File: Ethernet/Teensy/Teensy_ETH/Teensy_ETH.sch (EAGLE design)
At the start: 3 parts, among them M1 TEENSY4.1

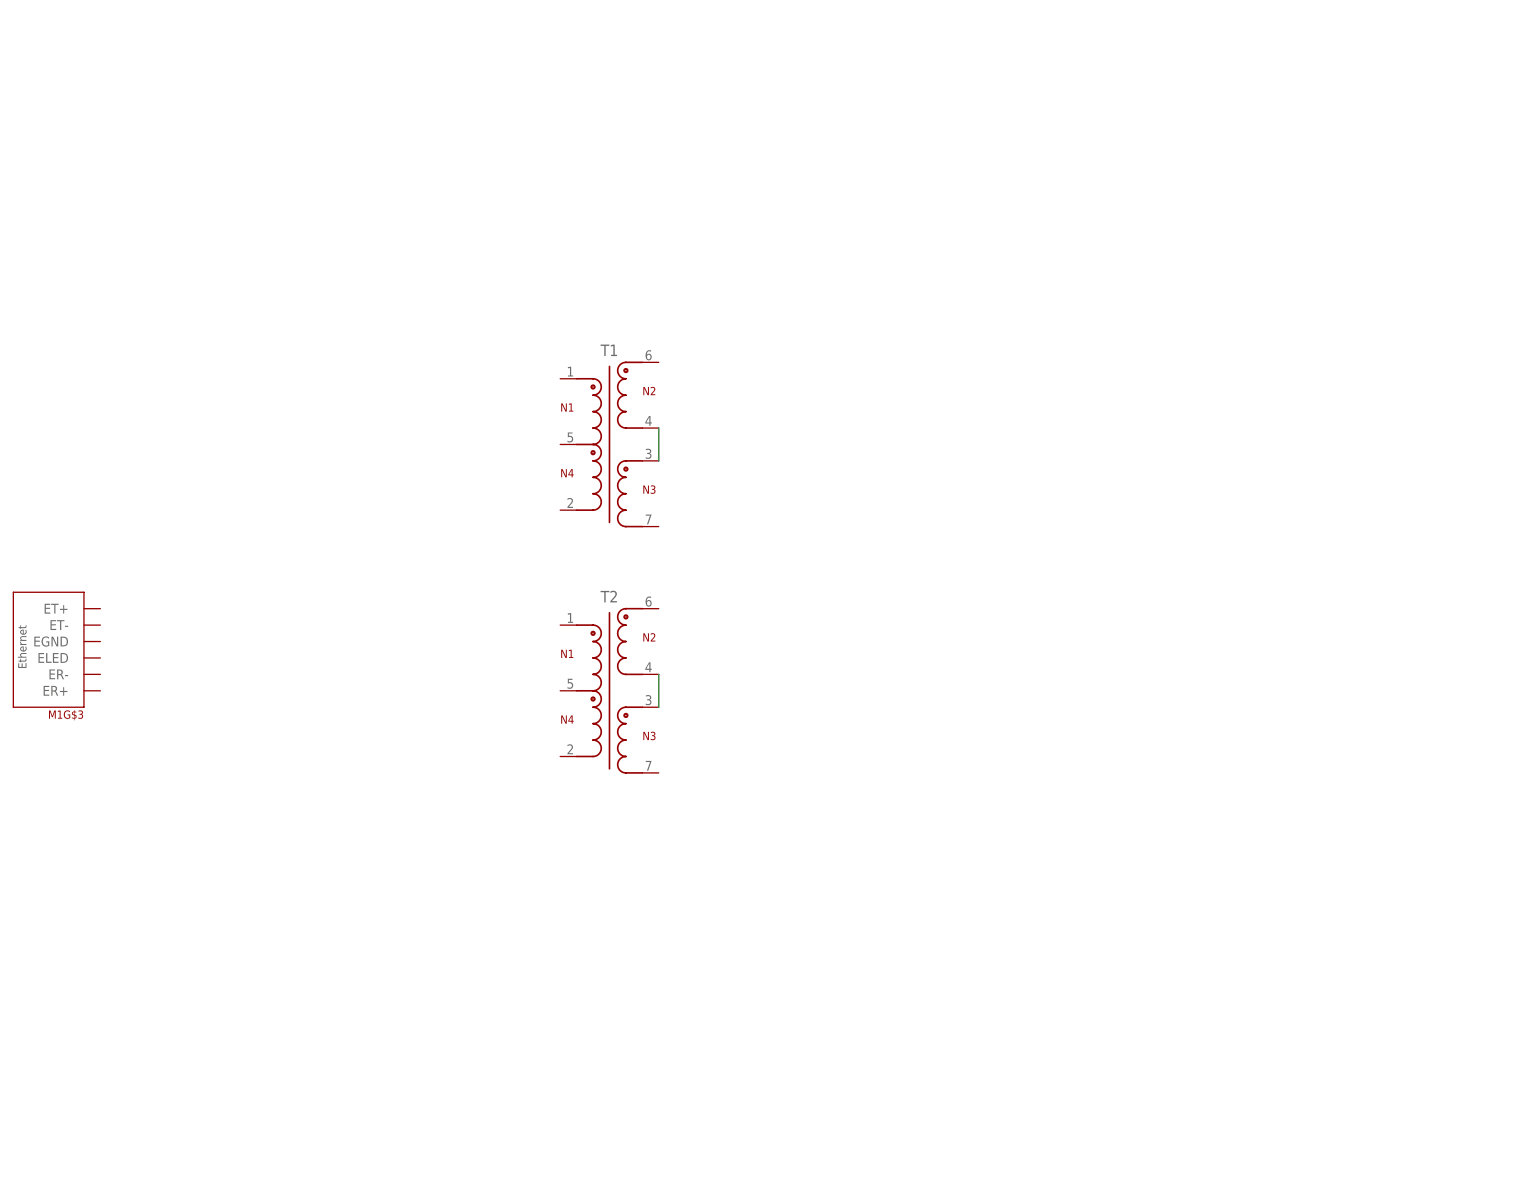
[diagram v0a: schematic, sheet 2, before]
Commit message: sicherung
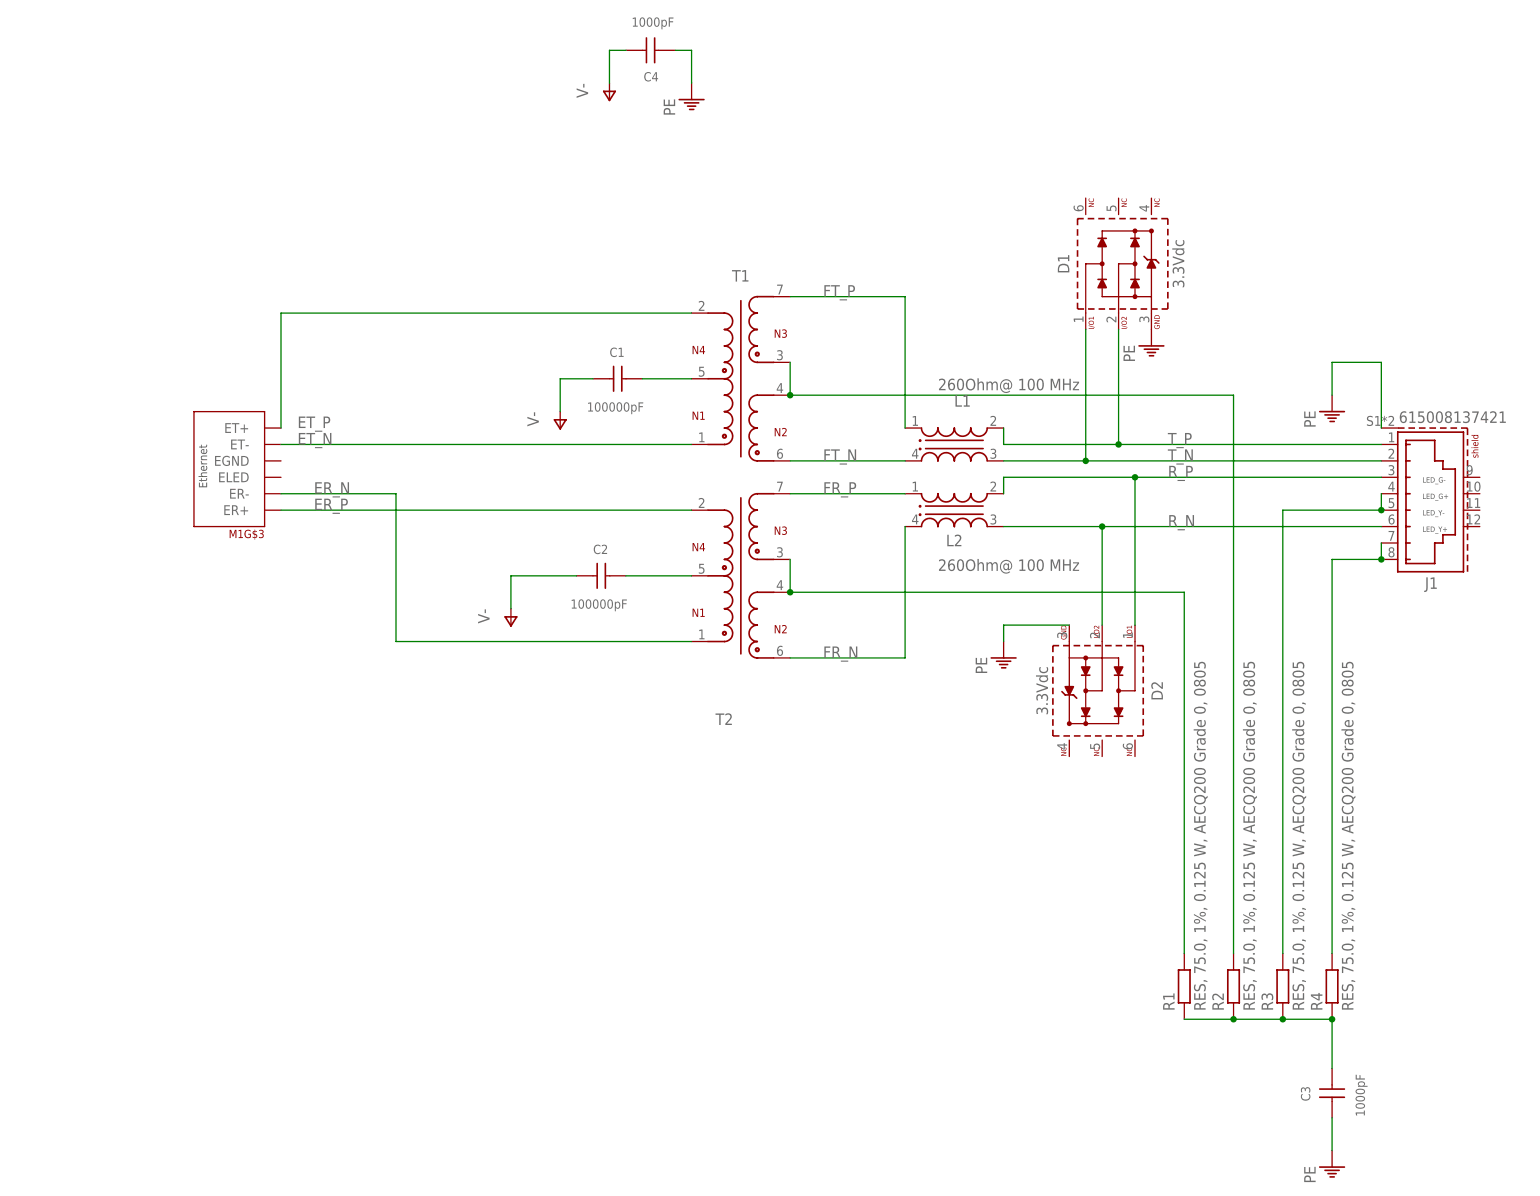
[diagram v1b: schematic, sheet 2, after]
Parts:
- added C1, C2: 100000pF, Wurth_Capacitors_WCAP-CSST:WCAP-CSST_0603_885382206004_R
- added C3, C4: 1000pF, Wurth_Capacitors_WCAP-CSMH:WCAP-CSMH_1206_H1.6_885342208024
- added D1, D2: 3.3Vdc, Wurth_EMC Components_WE-TVS:WE-TVS-SS_DFN1210-6L_824012823
- added J1: 615008137421, Wurth_Connectors_WR-MJ:615008137421
- added L1, L2: 260Ohm@ 100 MHz, Wurth_EMC Components_WE-CNSW:WE-CNSW_0805_744231261
- added R1, R2, R3, R4: RES, 75.0, 1%, 0.125 W, AECQ200 Grade 0, 0805, resistor:R-EU_R0805
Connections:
- new net ER_N: M1G$3.ER-, T2.1
- new net ER_P: M1G$3.ER+, T2.2
- new net ET_N: M1G$3.ET-, T1.1
- new net ET_P: M1G$3.ET+, T1.2
- new net FR_N: L2.1, T2.6
- new net FR_P: L2.4, T2.7
- new net FT_N: L1.1, T1.6
- new net FT_P: L1.4, T1.7
- new net N$17: C1.2, T1.5
- new net N$18: C2.2, T2.5
- new net N$19: C3.2, R1.1, R2.1, R3.1, R4.1
- new net N$7: J1.4, J1.5, R3.2
- new net N$8: J1.7, J1.8, R4.2
- new net PE: C3.1, C4.1, D1.GND, D2.GND, J1.SHIELD
- new net R_N: D2.I/O2, J1.6, L2.2
- new net R_P: D2.I/O1, J1.3, L2.3
- new net T_N: D1.I/O1, J1.2, L1.2
- new net T_P: D1.I/O2, J1.1, L1.3
- new net V-: C1.1, C2.1, C4.2
- net N$1: now also R2.2
- net N$2: now also R1.2
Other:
- moved on the sheet: M1G$3, T1, T2
